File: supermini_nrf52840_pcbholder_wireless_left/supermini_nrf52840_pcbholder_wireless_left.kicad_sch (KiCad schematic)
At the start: 9 parts, among them J1 Conn_01x07_Pin, J2 Conn_01x02_Pin, J3 Conn_01x07_Pin, J4 Conn_01x04_Pin, SW1 SW_SPDT, SW2 SW_SPST, U1 nice_nano

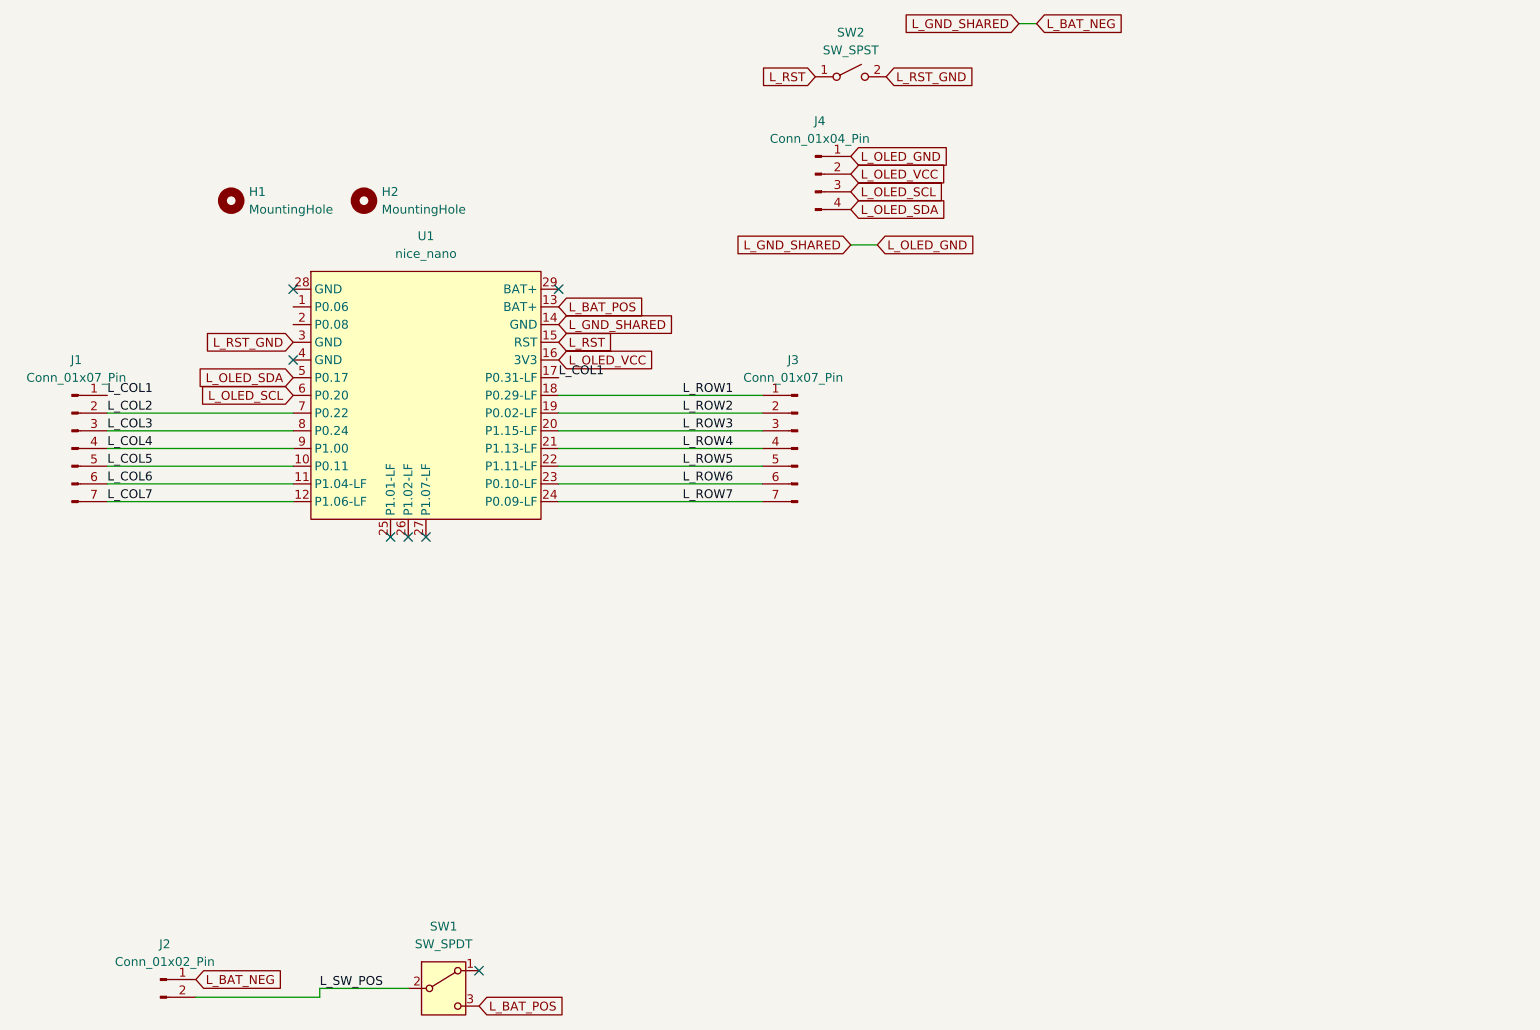
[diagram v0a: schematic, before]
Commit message: create left side and tweaks
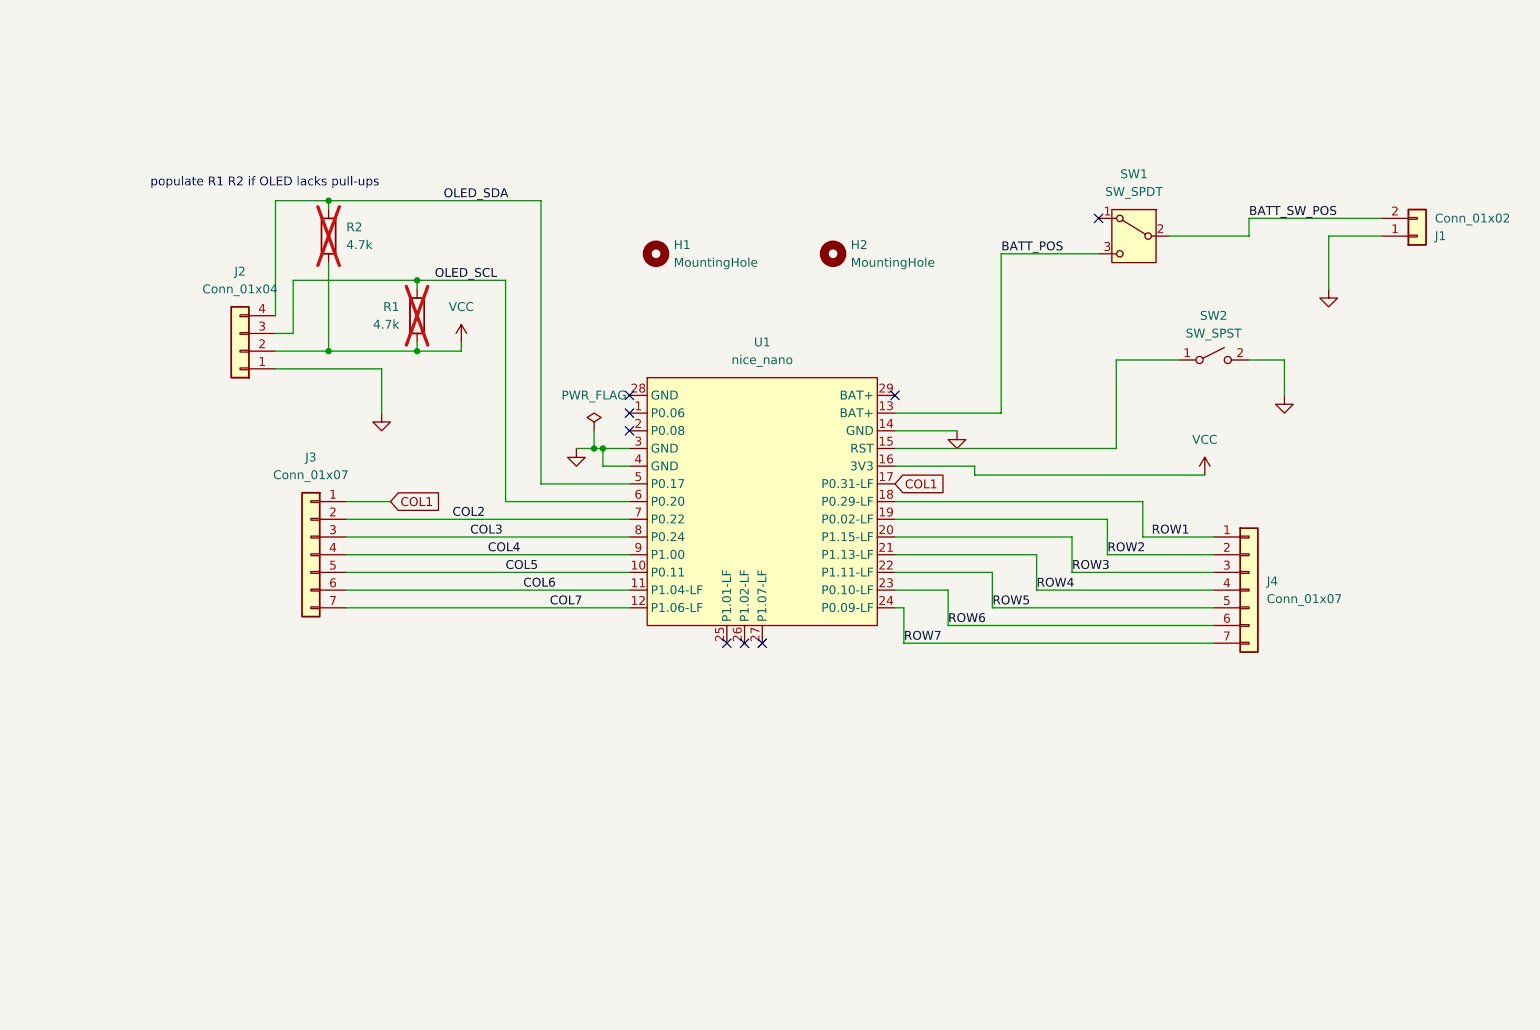
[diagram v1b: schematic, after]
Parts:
- removed J1, J3: Conn_01x07_Pin, Connector_PinHeader_2.54mm:PinHeader_1x07_P2.54mm_Vertical, symbol Connector:Conn_01x07_Pin
- removed J2: Conn_01x02_Pin, Connector_JST:JST_PH_S2B-PH-K_1x02_P2.00mm_Horizontal, symbol Connector:Conn_01x02_Pin
- removed J4: Conn_01x04_Pin, Connector_JST:JST_PH_S4B-PH-K_1x04_P2.00mm_Horizontal, symbol Connector:Conn_01x04_Pin
- added J1: Conn_01x02, Connector_JST:JST_PH_S2B-PH-K_1x02_P2.00mm_Horizontal, symbol Connector_Generic:Conn_01x02
- added J2: Conn_01x04, Connector_JST:JST_PH_S4B-PH-K_1x04_P2.00mm_Horizontal, symbol Connector_Generic:Conn_01x04
- added J3, J4: Conn_01x07, Connector_PinHeader_2.54mm:PinHeader_1x07_P2.54mm_Vertical, symbol Connector_Generic:Conn_01x07
- added R1, R2: 4.7k, Resistor_SMD:R_0805_2012Metric, symbol ScottoKeebs:Placeholder_Resistor
- H1, H2: footprint #footprint:M1.4_tapping_Hole_rev2 -> mounting-hole:M1.4_tapping_Hole_JLC
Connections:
- net L_BAT_NEG is gone; now on net GND: U1.14 (GND)
- net L_RST_GND is gone; now on net GND: SW2.2 (B), U1.3 (GND)
- net GND: now reaches U1.4 (GND)
- net GND: now also J1.1 (Pin_1), J2.1 (Pin_1)
- net L_BAT_POS renamed BATT_POS
- net L_COL1 renamed COL1
- net COL1: now also J3.1 (Pin_1)
- net L_COL2 renamed COL2
- net COL2: now also J3.2 (Pin_2)
- net L_COL3 renamed COL3
- net COL3: now also J3.3 (Pin_3)
- net L_COL4 renamed COL4
- net COL4: now also J3.4 (Pin_4)
- net L_COL5 renamed COL5
- net COL5: now also J3.5 (Pin_5)
- net L_COL6 renamed COL6
- net COL6: now also J3.6 (Pin_6)
- net L_COL7 renamed COL7
- net COL7: now also J3.7 (Pin_7)
- net L_OLED_SCL renamed OLED_SCL
- net OLED_SCL: now also J2.3 (Pin_3), R1.2
- net L_OLED_SDA renamed OLED_SDA
- net OLED_SDA: now also J2.4 (Pin_4), R2.2
- net L_OLED_VCC renamed VCC
- net VCC: now also J2.2 (Pin_2), R1.1, R2.1
- net L_ROW1 renamed ROW1
- net ROW1: now also J4.1 (Pin_1)
- net L_ROW2 renamed ROW2
- net ROW2: now also J4.2 (Pin_2)
- net L_ROW3 renamed ROW3
- net ROW3: now also J4.3 (Pin_3)
- net L_ROW4 renamed ROW4
- net ROW4: now also J4.4 (Pin_4)
- net L_ROW5 renamed ROW5
- net ROW5: now also J4.5 (Pin_5)
- net L_ROW6 renamed ROW6
- net ROW6: now also J4.6 (Pin_6)
- net L_ROW7 renamed ROW7
- net ROW7: now also J4.7 (Pin_7)
- net L_RST: no longer names the net of SW2.1 (A), U1.15 (RST)
- net L_SW_POS renamed BATT_SW_POS
- net BATT_SW_POS: now also J1.2 (Pin_2)
- no-connect marks 7 -> 8
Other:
- note added: "populate R1 R2 if OLED lacks pull-ups"
- title: (none) -> Left Dactyl Manuform Wireless Supermini nRF52840 Hub
